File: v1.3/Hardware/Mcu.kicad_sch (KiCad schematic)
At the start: 17 parts, among them J2 Conn_01x05, J5 Conn_01x08, U17 STM32F334C8Tx, Y1 8MHz

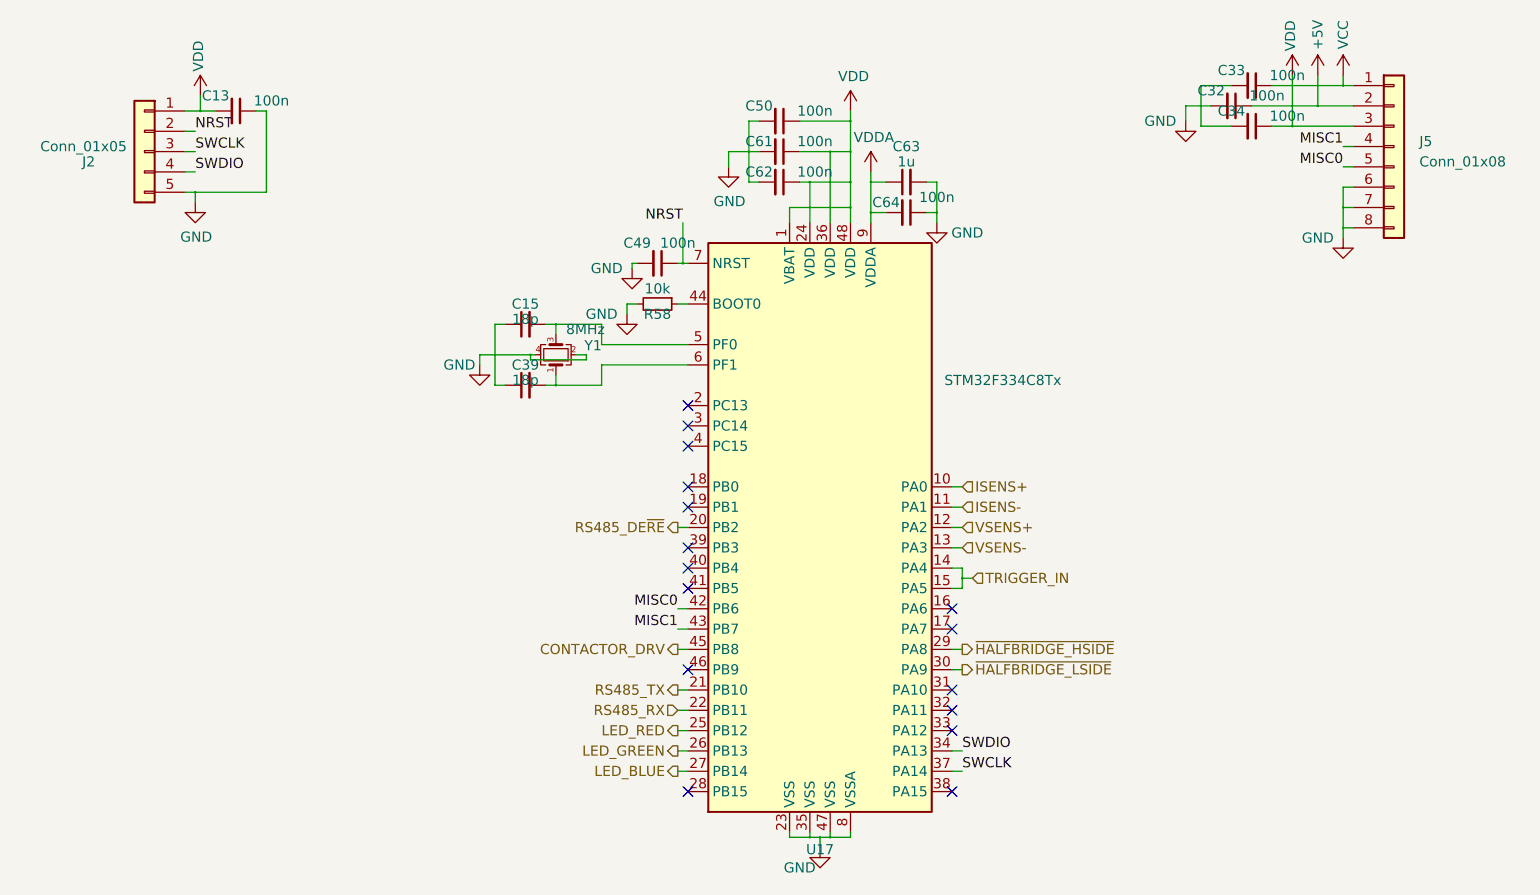
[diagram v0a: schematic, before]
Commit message: v1.3 Layout added & schematic update.
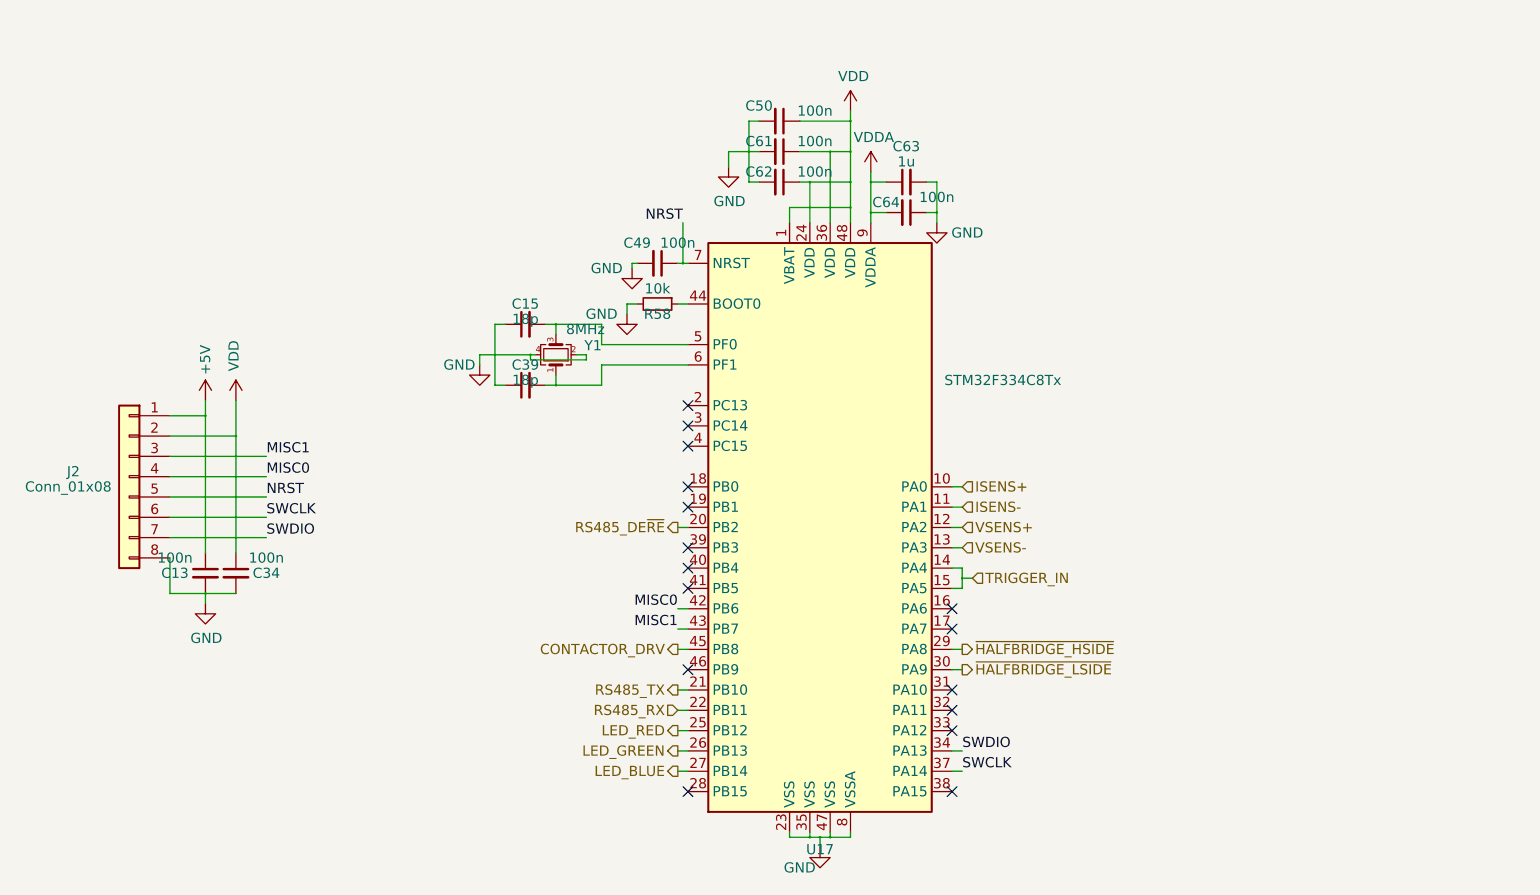
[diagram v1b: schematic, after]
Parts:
- removed C32, C33: 100n, Capacitor_SMD:C_0805_2012Metric, symbol Device:C_Small
- removed J2: Conn_01x05, Connector_PinHeader_2.54mm:PinHeader_1x05_P2.54mm_Vertical, symbol Connector_Generic:Conn_01x05
- removed J5: Conn_01x08, Connector_PinHeader_2.54mm:PinHeader_1x08_P2.54mm_Vertical, symbol Connector_Generic:Conn_01x08
- added J2: Conn_01x08, Connector_PinHeader_2.54mm:PinHeader_1x08_P2.54mm_Vertical, symbol Connector_Generic:Conn_01x08
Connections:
- net +5V: now also C13.1, J2.1 (Pin_1)
- net GND: now also C13.2, J2.8 (Pin_8); no longer C13.1
- net MISC0: now also J2.4 (Pin_4)
- net MISC1: now also J2.3 (Pin_3)
- net NRST: now also J2.5 (Pin_5)
- net SWCLK: now also J2.6 (Pin_6)
- net SWDIO: now also J2.7 (Pin_7)
- net VDD: now also J2.2 (Pin_2); no longer C13.2
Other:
- moved on the sheet: C13, C34
